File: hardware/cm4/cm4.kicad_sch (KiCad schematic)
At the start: 15 parts, among them J11 CM4 Stecker 1, J12 CM4 Stecker 2, M1 Raspberry Pi CM4 (z. B. CM410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, Q10 BSS84

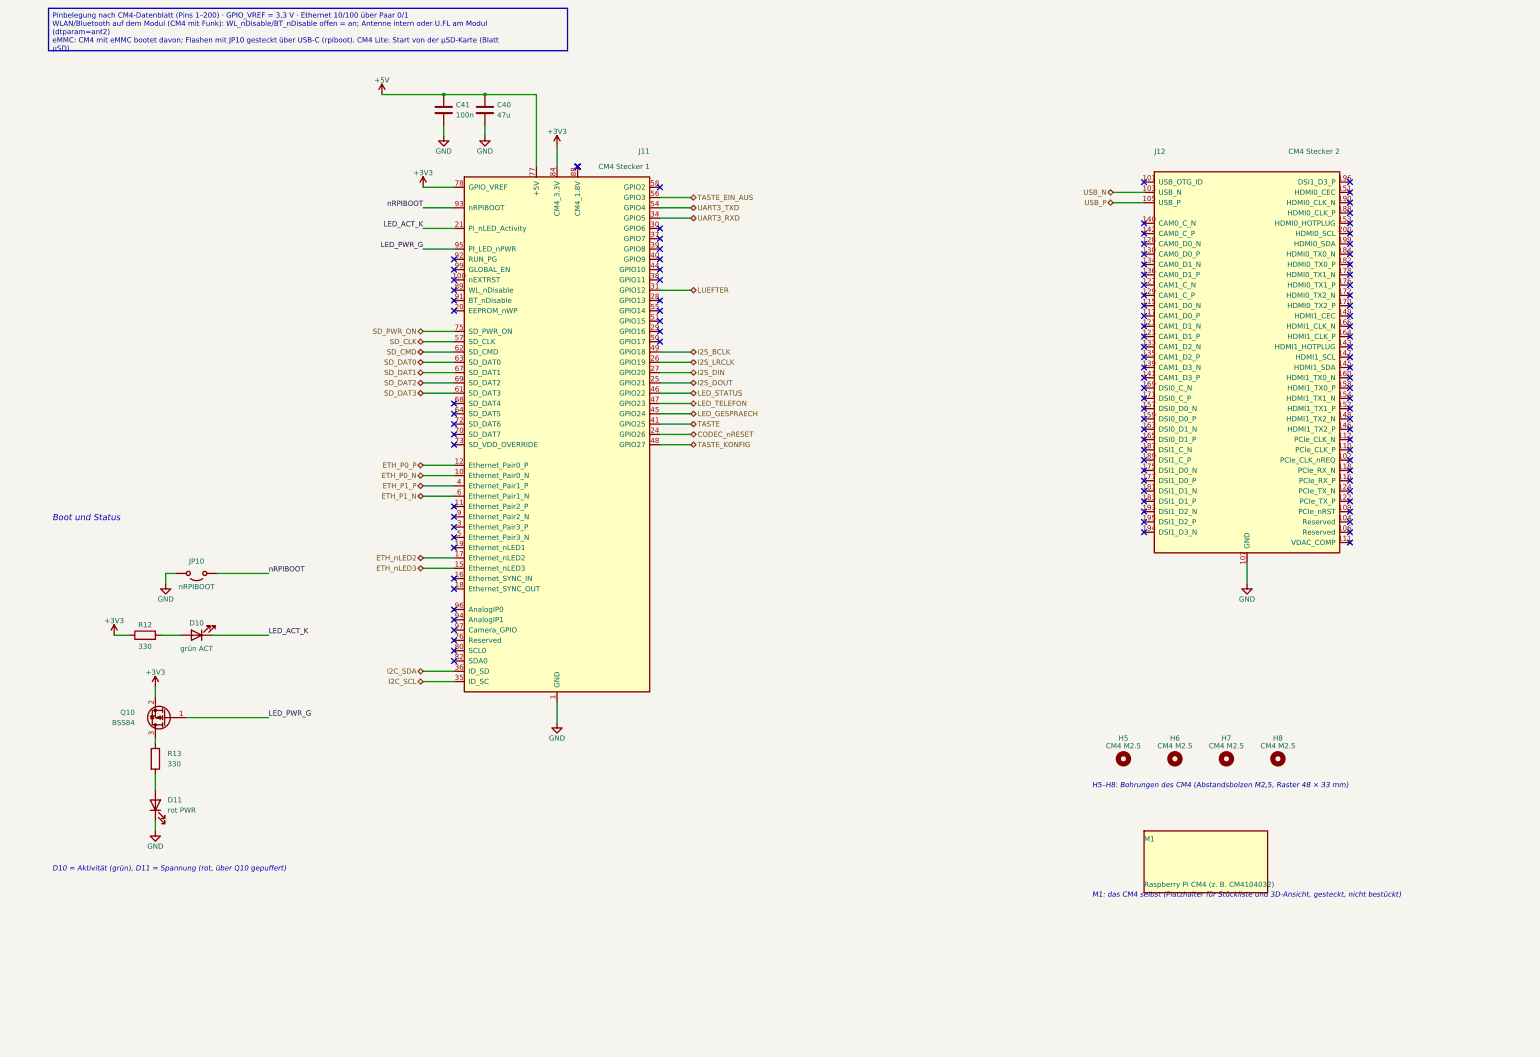
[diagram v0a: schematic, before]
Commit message: CM4-Schaltplan: Handänderungen übernommen (Handlage für 8 Blätter, 2 Texte zurückgeführt); Kastenhöhen aus gemessenen Zeichenbreiten
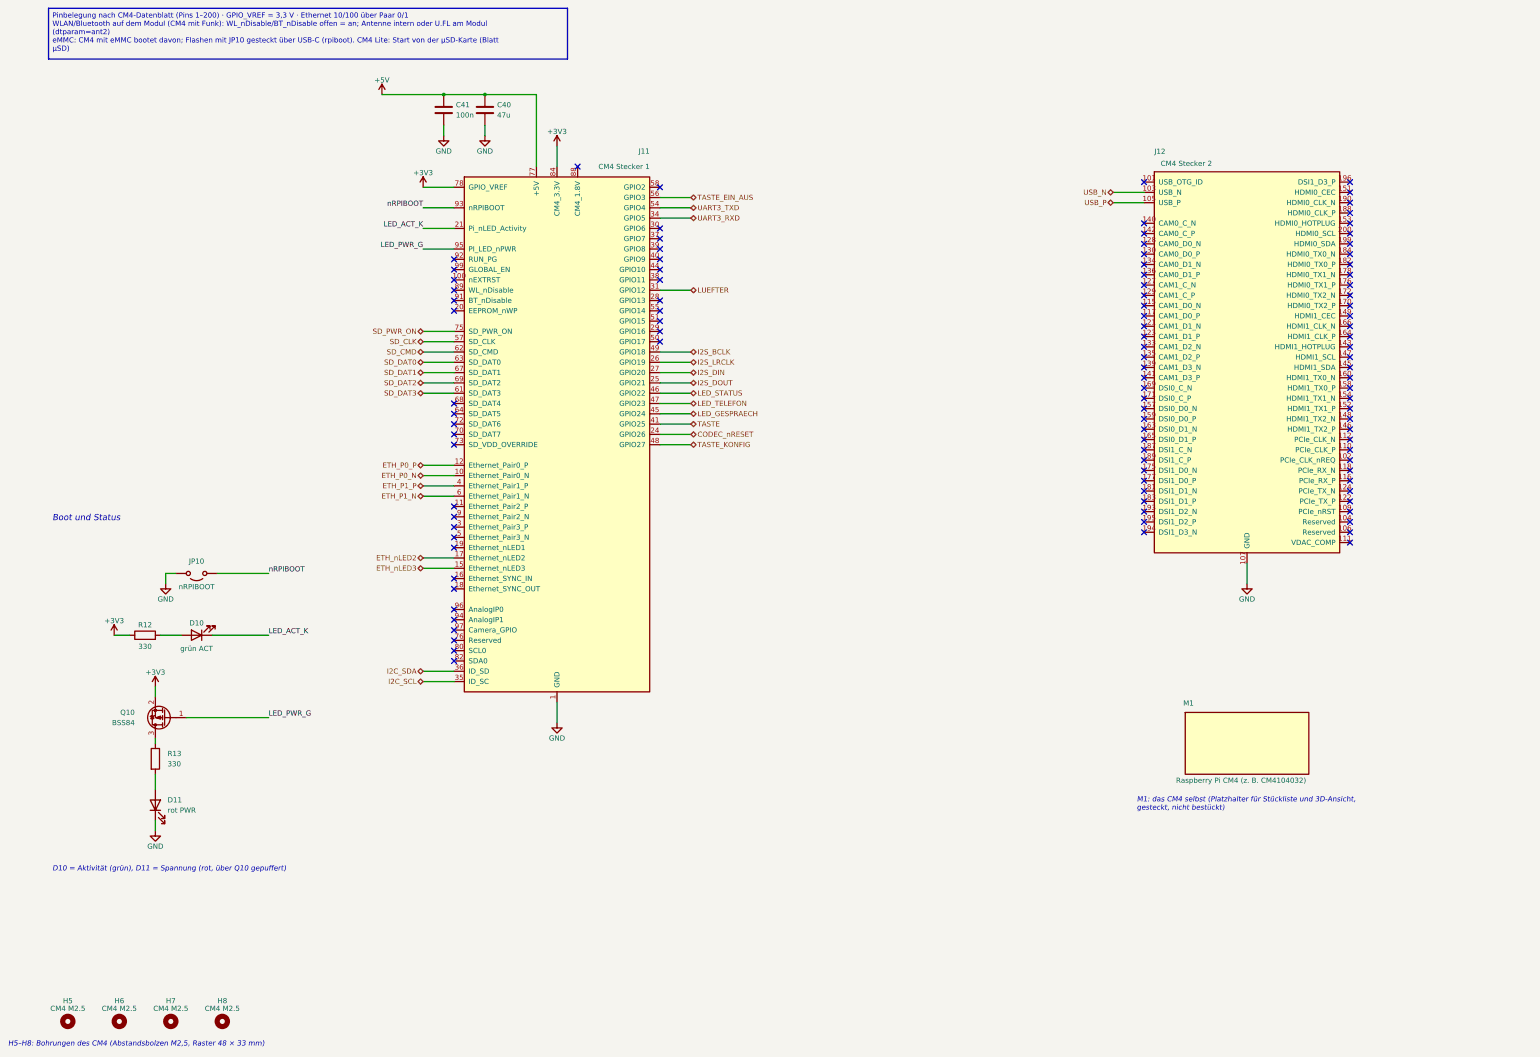
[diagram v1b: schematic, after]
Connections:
- no-connect marks 107 -> 105
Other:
- moved on the sheet: H5, H6, H7, H8, M1
